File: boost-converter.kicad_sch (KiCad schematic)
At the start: 1 part, among them U2 LM5122ZPWPR

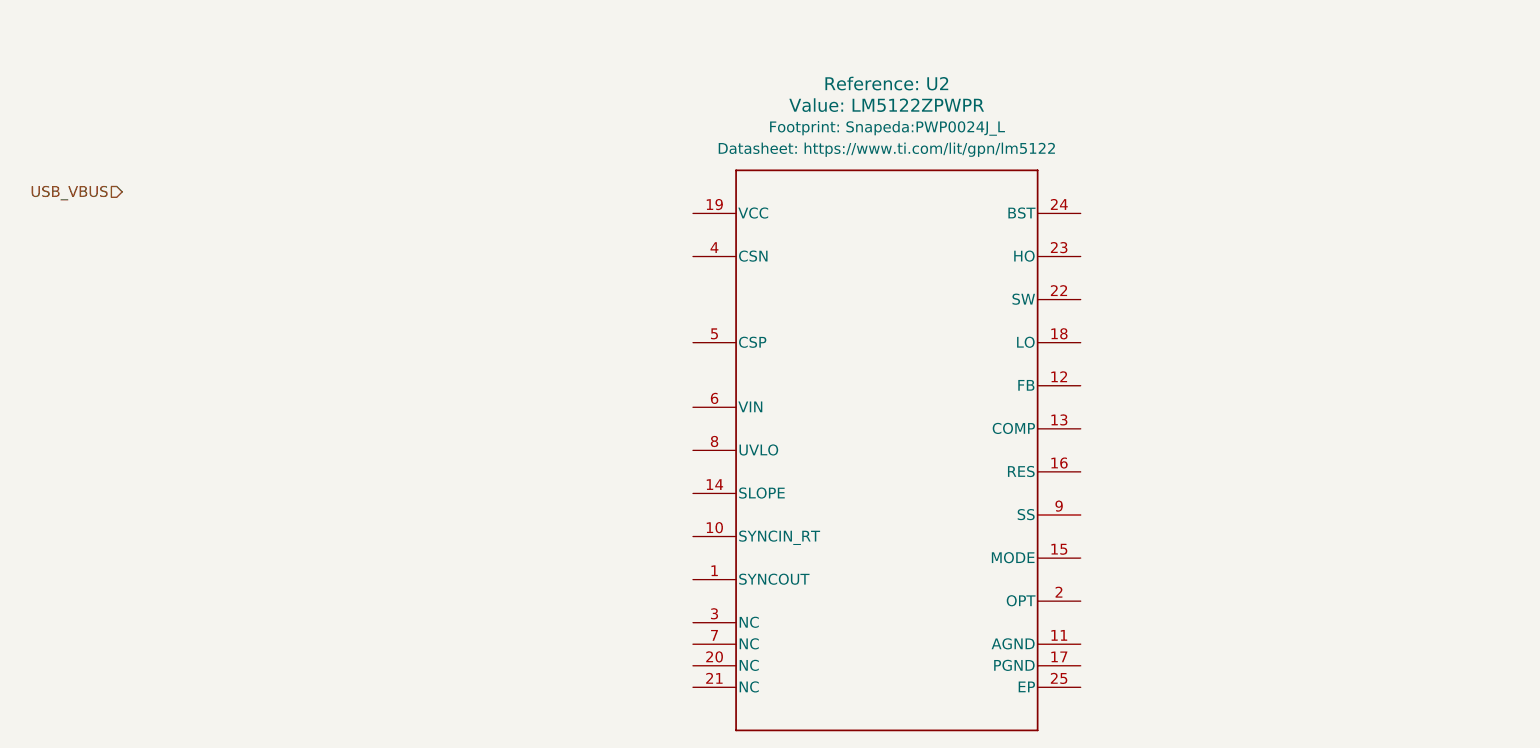
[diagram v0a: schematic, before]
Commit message: syncing
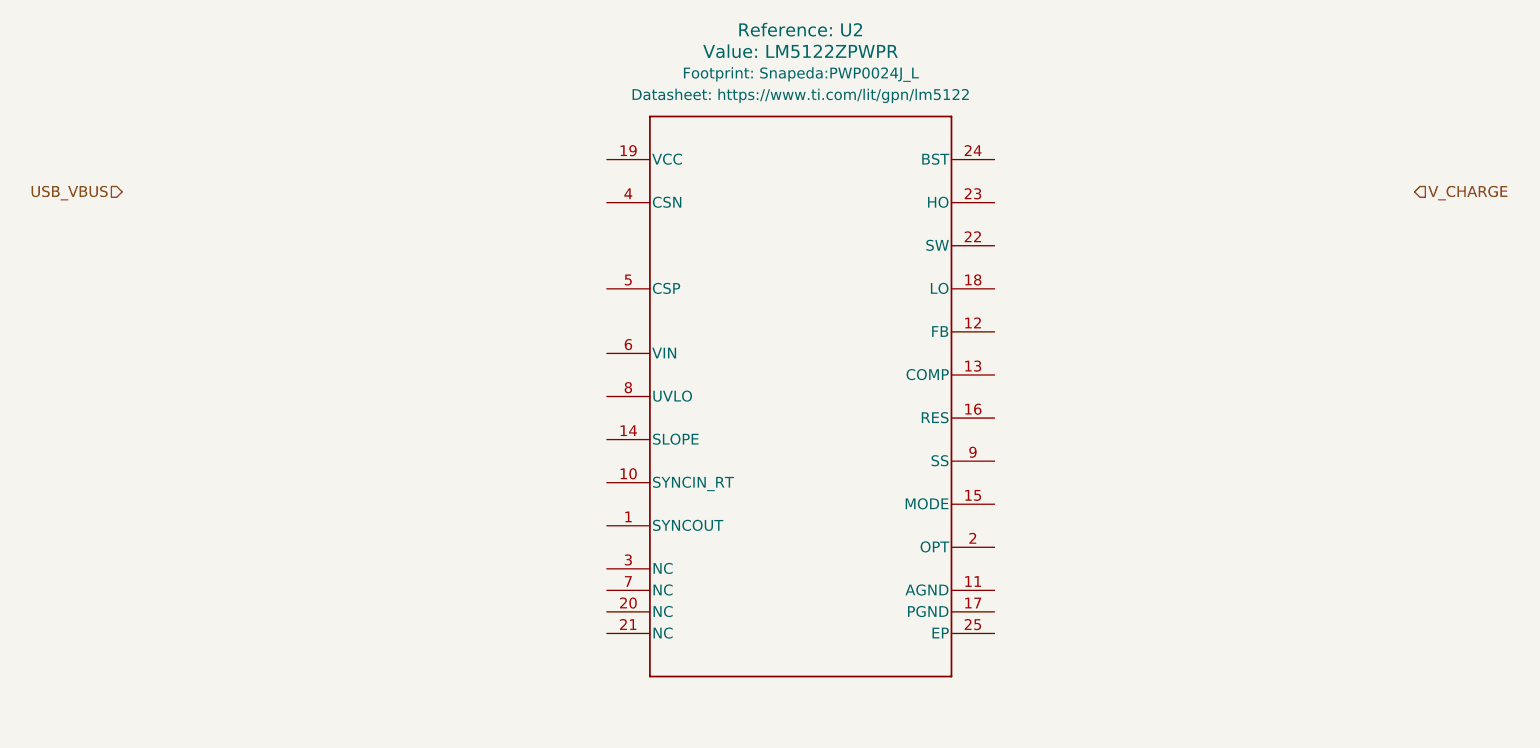
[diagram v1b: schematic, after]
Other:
- moved on the sheet: Reference: U2
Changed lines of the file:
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@@
+		)
+	)
+	(hierarchical_label "V_CHARGE"
+		(shape input)
+		(at 203.2 63.5 0)
+		(effects
+			(font
+				(size 1.27 1.27)
+			)
+			(justify left)
 		)
 	)
 	(symbol
 		(lib_id "Snapeda:LM5122ZPWPR")
-		(at 140.97 93.98 0)
+		(at 130.81 87.63 0)
 		(unit 1)
 		(body_style 1)
@@
 		(fields_autoplaced yes)
 		(property "Reference" "U2"
-			(at 140.97 50.8 0)
+			(at 130.81 44.45 0)
 			(show_name yes)
 			(do_not_autoplace no)
@@
 		)
 		(property "Value" "LM5122ZPWPR"
-			(at 140.97 53.34 0)
+			(at 130.81 46.99 0)
 			(show_name yes)
 			(do_not_autoplace no)
@@
 		)
 		(property "Footprint" "Snapeda:PWP0024J_L"
-			(at 140.97 55.88 0)
+			(at 130.81 49.53 0)
 			(show_name yes)
 			(do_not_autoplace no)
@@
 		)
 		(property "Datasheet" "https://www.ti.com/lit/gpn/lm5122"
-			(at 140.97 58.42 0)
+			(at 130.81 52.07 0)
 			(show_name yes)
 			(do_not_autoplace no)
@@
 		)
 		(property "Description" ""
-			(at 140.97 93.98 0)
+			(at 130.81 87.63 0)
 			(show_name yes)
 			(do_not_autoplace no)

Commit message: added boost converter schematic
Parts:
- removed U2: LM5122ZPWPR, Snapeda:PWP0024J_L, symbol Snapeda:LM5122ZPWPR
- added C12: 100pF, symbol Device:C
- added Cboot1: 100nF, symbol Device:C
- added Ccomp1: 470nF, symbol Device:C
- added Ccomp1: 8.2nF, symbol Device:C
- added Cin1, Cvcc1: 10uF, symbol Device:C
- added Cout1: 22uF, symbol Device:C
- added Css1: 4.7nF, symbol Device:C
- added Cvin1: 100nF/50V, symbol Device:C
- added Dboot1: 700mV, symbol Device:D_Schottky
- added L1: 8.2uH/14.5mR, Inductor_SMD:L_Coilcraft_XAL7070-XXX, symbol Device:L
- added Q1, Q2: CSD18543Q3A, Package_SON:VSON-8_3.3x3.3mm_P0.65mm_NexFET, symbol Transistor_FET:CSD18543Q3A
- added R13, R14: 10R, symbol Device:R
- added Rcomp1: 4.87kR, symbol Device:R
- added Rfbb1, Rfbt1: R, symbol Device:R
- added Rpg1: 10k, symbol Device:R
- added Rsns1, Rsns2: 8mR, Resistor_SMD:R_0612_1632Metric, symbol Device:R
- added Rt1: 110k, symbol Device:R
- added U2: TPS43060RTER, Package_DFN_QFN:Texas_RTE_WQFN-16-1EP_3x3mm_P0.5mm_EP1.2x0.8mm, symbol Snapeda:TPS43060RTER
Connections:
- net USB_VBUS: now also Cin1.1, Cvin1.2, R13.2, Rsns1.1, Rsns2.1, U2.7 (VIN)
- net V_CHARGE: now also Cout1.1, Q2.5 (D), Rfbt1.1
- new net: Rpg1.1, U2.14 (PGOOD)
- new net: Ccomp1.2, Rcomp1.1
- new net: Ccomp1.2, Rcomp1.2, U2.3 (COMP)
- new net: Rt1.2, U2.1 (RT/CLK)
- new net: Css1.2, U2.2 (SS)
- new net: L1.1, R14.2, Rsns1.2, Rsns2.2
- new net BOOT: Cboot1.2, Dboot1.1 (K), U2.11 (BOOT)
- new net FB: Rfbb1.1, Rfbt1.2, U2.4 (FB)
- new net GND: Ccomp1.1, Ccomp1.1, Cin1.2, Cout1.2, Css1.1, Cvcc1.2, Cvin1.1, Q1.1 (S), Q1.2 (S), Q1.3 (S), Rfbb1.2, Rt1.1, U2.16 (AGND_16), U2.17 (AGND_17), U2.9 (PGND)
- new net HDRV: Q2.4 (G), U2.13 (HDRV)
- new net ISNS+: C12.1, R13.1, U2.6 (ISNS+)
- new net ISNS-: C12.2, R14.1, U2.5 (ISNS-)
- new net LDRV: Q1.4 (G), U2.8 (LDRV)
- new net SW: Cboot1.1, L1.2, Q1.5 (D), Q2.1 (S), Q2.2 (S), Q2.3 (S), U2.12 (SW)
- new net VCC: Cvcc1.1, Dboot1.2 (A), Rpg1.2, U2.10 (VCC)
- no-connect marks 0 -> 1
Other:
- note added: "INPUT 20V ~5A (100W)"
- note added: "OUTPUT 42V@3A"
- note added: "bullfrog ENABLE PIN INTERNAL PULLUP. COULD CONNECT TO A SWITCH OR SOMETHING"
- note added: "https://webench.ti.com/appinfo/webench/scripts/SDP.cgi?ID=E0FB6AADAF190E80"
